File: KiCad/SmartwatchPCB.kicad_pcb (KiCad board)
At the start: 2 copper layers, 28.4 x 40 mm, 38 parts, among them IC1 SAML22G, IC2 TFBS4711, J1 USB_B_Micro, J2 Conn_01x04_Male, J3 Conn_01x04_Male, U1 LCD

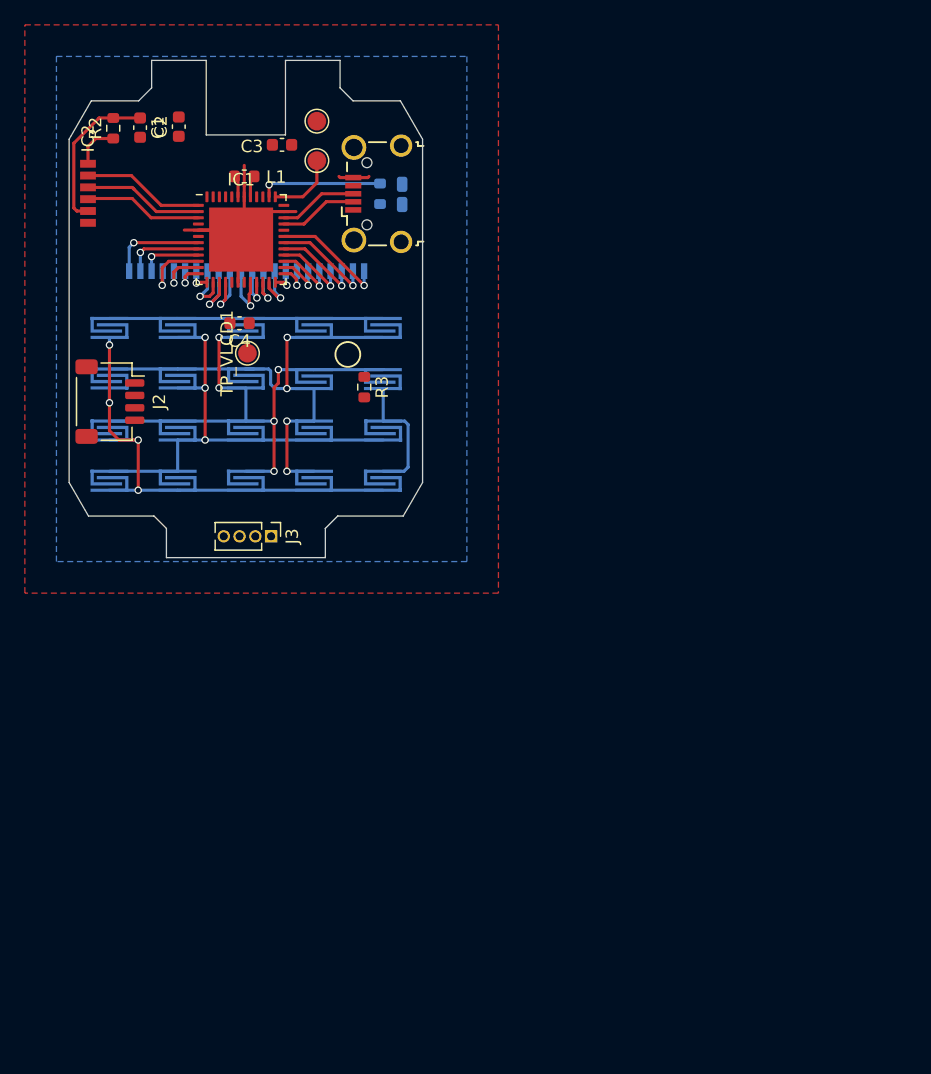
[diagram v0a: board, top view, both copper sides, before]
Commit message: close to ordering first version
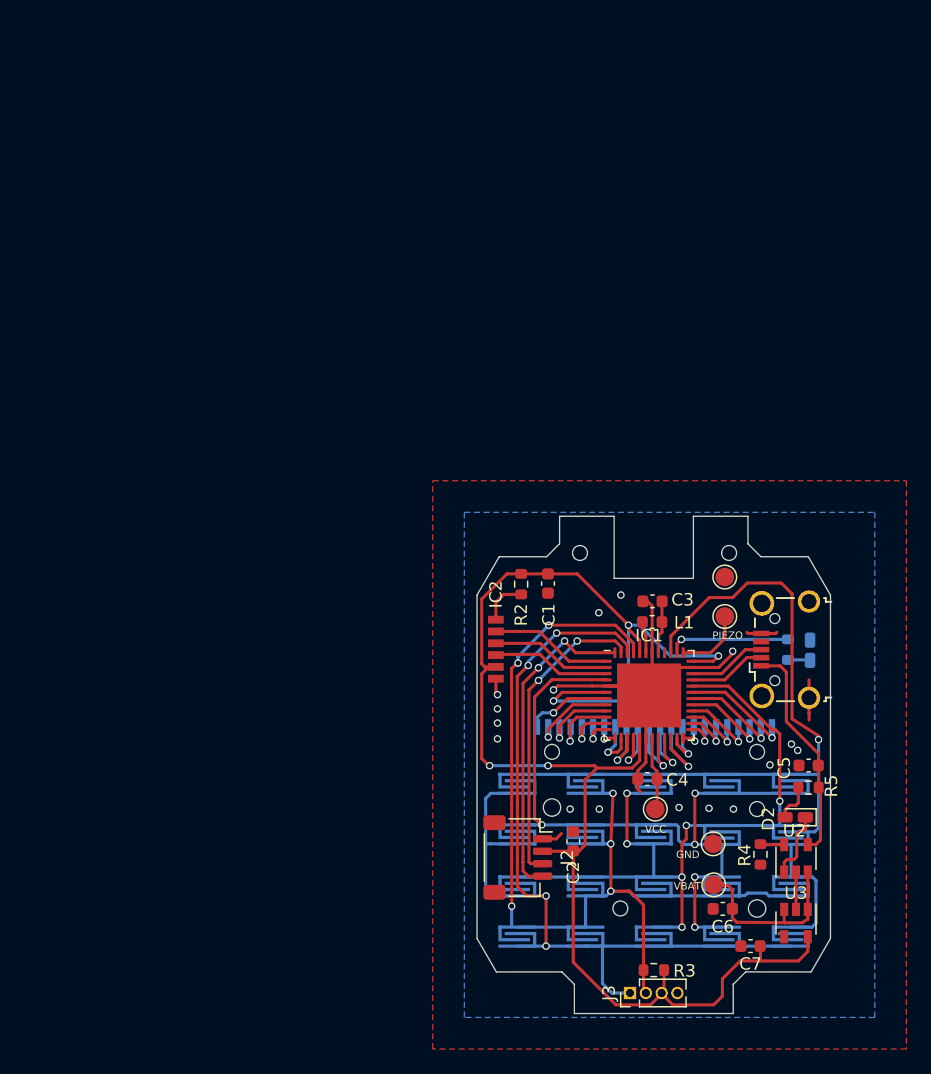
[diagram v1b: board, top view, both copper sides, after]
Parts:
- added C5: 100nF, Capacitor_SMD:C_0603_1608Metric, F.Cu at (45.3, 36.7)
- added C6: 100nF, Capacitor_SMD:C_0603_1608Metric, F.Cu at (38.4, 48.3)
- added C7: 100nF, Capacitor_SMD:C_0603_1608Metric, F.Cu at (40.6, 51.3)
- added D2: LED, LED_SMD:LED_0603_1608Metric_Castellated, F.Cu at (44.2, 40.9)
- added R4: R, Resistor_SMD:R_0603_1608Metric, F.Cu at (41.4, 43.9)
- added R5: R, Resistor_SMD:R_0603_1608Metric, F.Cu at (45.3, 38.5)
- added TP_GND1: TestPoint, TestPoint:TestPoint_Pad_D1.5mm, F.Cu at (37.6, 43.0)
- added TP_VBAT1: TestPoint, TestPoint:TestPoint_Pad_D1.5mm, F.Cu at (37.6, 46.3)
- added U2: MCP73831-2-OT, Package_TO_SOT_SMD:SOT-23-5, F.Cu at (44.3, 44.2)
- added U3: AP2112K-2.5, Package_TO_SOT_SMD:SOT-23-5, F.Cu at (44.3, 49.4)
- U1: footprint SmartwatchPCB:display -> SmartwatchPCB:display_MOUNT
- moved C2 65.7 mm to (26.3, 42.8)
- moved R3 52.4 mm to (32.8, 53.2), turned to 180 degrees
- moved TP_VLCD1 49.2 mm to (32.9, 40.2)
- moved U1 49.2 mm to (32.9, 33.6)
- moved C1 49.2 mm to (24.3, 22.1)
- moved C4 49.2 mm to (32.3, 37.8)
- moved D1 49.2 mm to (45.4, 27.5)
- moved IC1 49.2 mm to (32.4, 31.1)
- moved IC2 49.2 mm to (20.1, 27.4)
- moved J1 49.2 mm to (43.4, 27.4)
- moved J2 49.2 mm to (21.9, 44.1)
- moved R1 49.2 mm to (43.6, 27.4)
- moved R2 49.2 mm to (22.1, 22.1)
- moved SW_0 49.2 mm to (38.3, 50.5)
- moved SW_1 49.2 mm to (38.3, 46.5)
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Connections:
- J1 pad 1: Net-(J1-Pad1) -> VBUS
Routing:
- net VCC: track 12.6 -> 120.4 mm, vias 0 -> 5
- net SWCLK: track 37.2 -> 79.9 mm, vias 3 -> 6
- net SWDIO: track 39.7 -> 80.3 mm
- net KEYPAD_1: track 32.4 -> 69.0 mm, vias 0 -> 1
- net SCL: track 0.00 -> 26.1 mm, vias 0 -> 2
- net SDA: track 0.00 -> 24.6 mm, vias 0 -> 2
- net GND: track 12.8 -> 35.1 mm, vias 0 -> 15
- net VBUS: track 0.00 -> 18.1 mm
- net KEYPAD_2: track 41.2 -> 58.3 mm, vias 4 -> 5
- net KEYPAD_3: track 43.3 -> 59.4 mm, vias 5 -> 6
- net VBAT: track 0.00 -> 15.1 mm
- net VCC_LCD: track 0.00 -> 5.92 mm
- net Net-(D2-Pad1): track 0.00 -> 5.62 mm
- net Net-(D2-Pad2): track 0.00 -> 3.08 mm
- net Net-(IC1-Pad22): track 3.76 -> 6.62 mm
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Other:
- outline, holes or cut-outs redrawn
- board text added: "GND"
- board text added: "PIEZO"
- board text added: "VBAT"
- board text added: "VCC"
